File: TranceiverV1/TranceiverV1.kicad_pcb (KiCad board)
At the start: 2 copper layers, 4 parts, among them J1 Conn_01x03_Socket, J3 Conn_01x02_Socket, J5 Conn_02x04_Odd_Even, U3 102010388

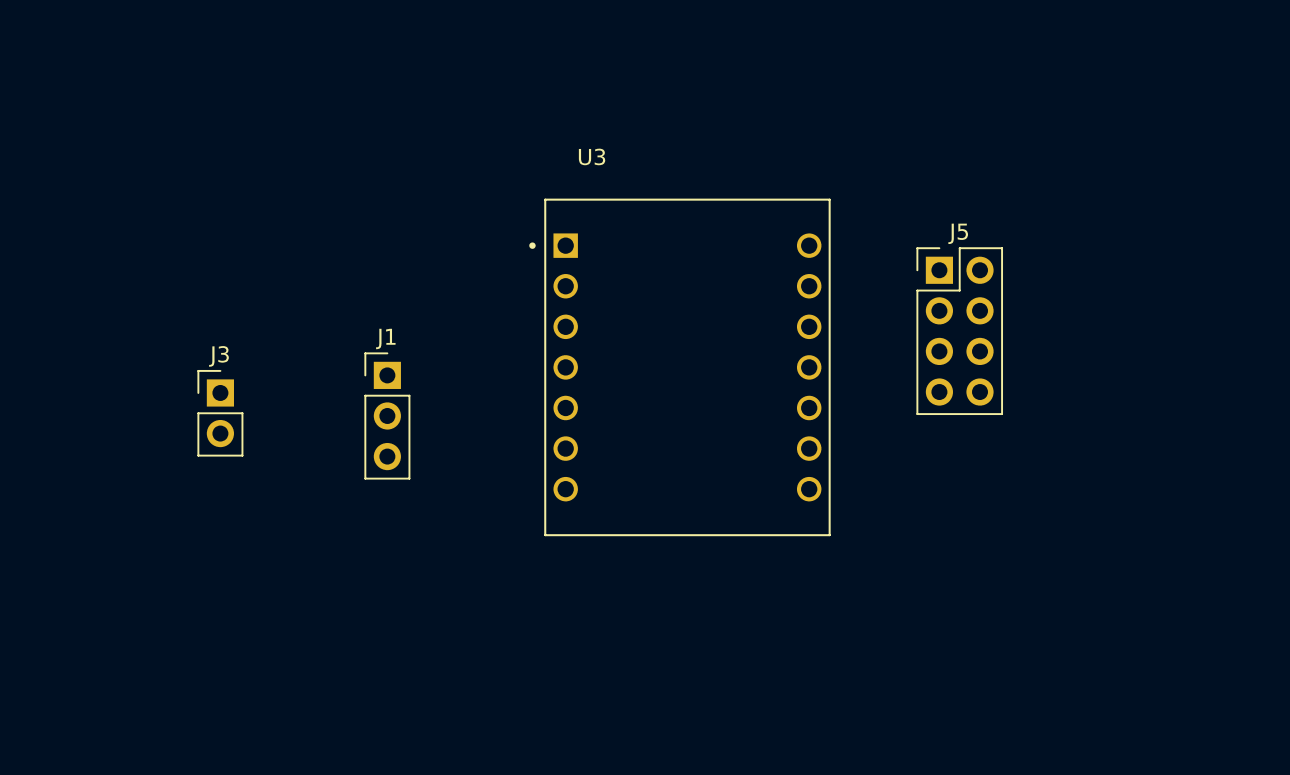
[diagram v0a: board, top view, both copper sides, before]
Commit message: designed first iteration of pcb
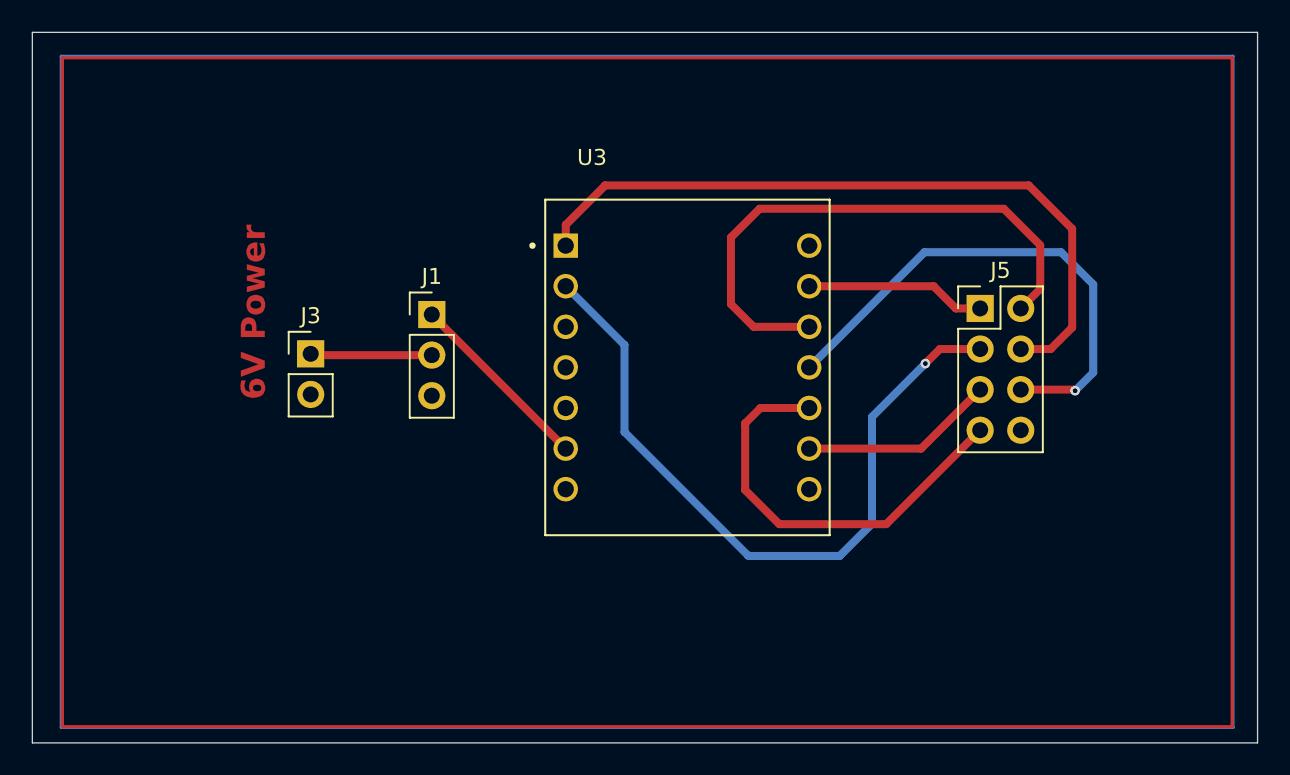
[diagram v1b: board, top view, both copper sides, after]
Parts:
- moved J3 6.16 mm to (150.4, 124.2)
- moved J1 4.72 mm to (158.0, 121.7)
- moved J5 3.49 mm to (192.3, 121.3)
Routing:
- net /CE: track 0.00 -> 45.4 mm, vias 0 -> 1
- net /CS: track 0.00 -> 45.1 mm
- net /VCC: track 0.00 -> 35.2 mm
- net /MOSI: track 0.00 -> 32.2 mm, vias 0 -> 1
- net /MISO: track 0.00 -> 26.6 mm
- net /SCK: track 0.00 -> 12.2 mm
- net /SERVO_DATA: track 0.00 -> 11.9 mm
- net GND: track 0.00 -> 11.3 mm
- net Net-(J1-Pin_2): track 0.00 -> 7.61 mm
- added copper zone on B.Cu, net GND
- added copper zone on F.Cu, net GND
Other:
- board outline added: 76.7 x 44.5 mm
- board text added: "6V Power"
